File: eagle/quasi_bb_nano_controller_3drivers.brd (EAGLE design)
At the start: 62.4 x 70.6 mm, 10 parts, among them X1 JST-XH-08-PIN-LONG-PAD, X2 JST-XH-08-PIN-LONG-PAD, X3 JST-XH-02-PIN-LONG-PAD, X4 JST-XH-08-PIN-LONG-PAD, X5 JST-XH-08-PIN-LONG-PAD

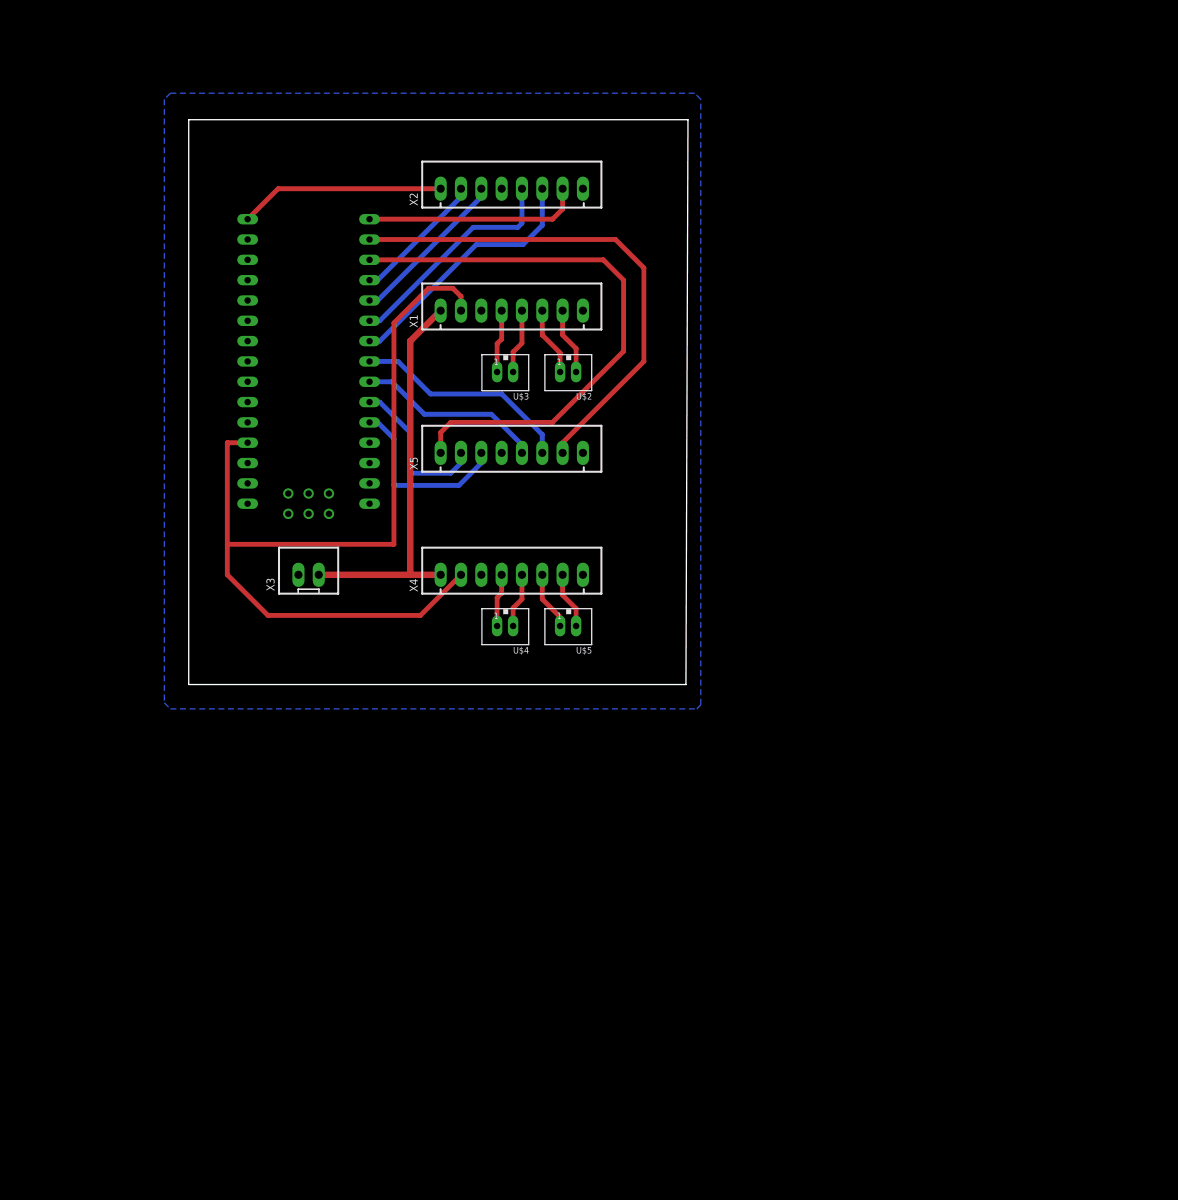
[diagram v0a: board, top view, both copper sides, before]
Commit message: Add eagle
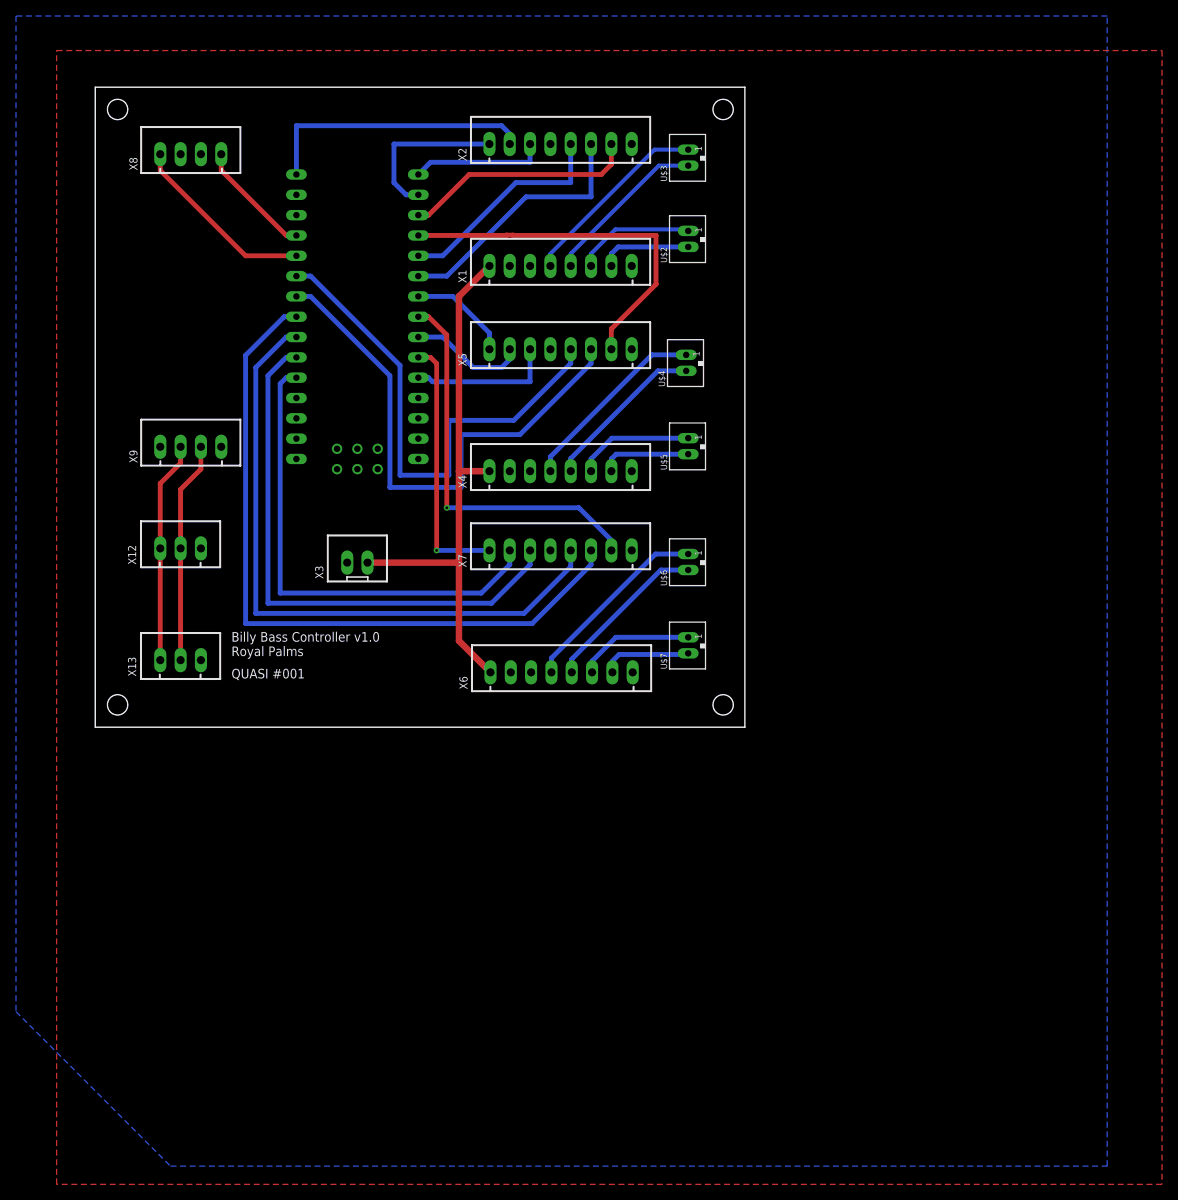
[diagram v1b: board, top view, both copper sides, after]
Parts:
- added U$6, U$7: JST-PH_2-PIN_HEADER, con-jst-ph:JST_B2B-PH_HEADER
- added X12, X13: JST-XH-03-PIN-LONG-PAD, Rembrandt Electronics - JST XH Connectors v1-0:JST-XH-03-PACKAGE-LONG-PAD
- added X6, X7: JST-XH-08-PIN-LONG-PAD, Rembrandt Electronics - JST XH Connectors v1-0:JST-XH-08-PACKAGE-LONG-PAD
- added X8, X9: JST-XH-04-PIN-LONG-PAD, Rembrandt Electronics - JST XH Connectors v1-0:JST-XH-04-PACKAGE-LONG-PAD
- moved U$4 39.8 mm to (73.9, 45.5), turned to 90 degrees
- moved U$3 35.1 mm to (74.2, 71.1), turned to 90 degrees
- moved U$5 26.9 mm to (74.2, 35.1), turned to 90 degrees
- moved U$2 22.3 mm to (74.2, 61.0), turned to 90 degrees
- moved X5 14.3 mm to (58.2, 47.2)
- moved X4 14.3 mm to (58.2, 32.0)
- moved U$1 8.27 mm to (35.3, 42.4)
- moved X1 8.27 mm to (58.2, 57.7)
- moved X2 8.27 mm to (58.2, 72.9)
- moved X3 6.28 mm to (32.8, 20.6)
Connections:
- removed net N$12: X2.4
- removed net N$121: X5.4
- new net 485_A: X12.1, X13.1, X9.2
- new net 485_B: X12.2, X13.2, X9.3
- new net A0: U$1.A0, X8.4
- new net A01_2: U$6.P1, X6.4
- new net A02_2: U$6.P2, X6.5
- new net A1: U$1.A1, X8.1
- new net A1_2: U$1.A6, X7.3
- new net A2_2: U$1.A7, X7.2
- new net B01_2: U$7.P2, X6.7
- new net B02_2: U$7.P1, X6.6
- new net B1_2: U$1.A5, X7.5
- new net B2_2: U$1.A4, X7.6
- new net PWMA_2: U$1.D3, X7.1
- new net PWMB_2: U$1.D5, X7.7
- net A1_0: now also U$1.D12; no longer U$1.D8
- net A2_0: now also U$1.D13; no longer U$1.D9
- net A2_1: now also U$1.D4; no longer U$1.D3
- net B1_0: now also U$1.D8; no longer U$1.D7
- net B1_1: now also U$1.A2; no longer U$1.D4
- net B2_0: now also U$1.D7; no longer U$1.D6
- net B2_1: now also U$1.A3; no longer U$1.D5
- net GND: now also X12.3, X13.3, X6.3, X6.8, X7.8, X8.2, X8.3, X9.1
- net PWMA_0: now also U$1.D11; no longer U$1.D13
- net PWMA_1: now also U$1.D6; no longer U$1.D10
- net PWMB_0: now also U$1.D10; no longer U$1.D12
- net PWMB_1: now also U$1.D9; no longer U$1.D11
- net VCC: now also X6.2, X9.4
- net VM: now also X6.1
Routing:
- net VCC: track 129.9 -> 0.00 mm
- net B2_2: track 0.00 -> 89.9 mm
- net B1_2: track 0.00 -> 81.2 mm
- net A1_2: track 0.00 -> 69.5 mm
- net A2_2: track 0.00 -> 60.5 mm
- net PWMA_1: track 71.3 -> 12.8 mm
- net PWMB_2: track 0.00 -> 49.6 mm, vias 0 -> 1
- net B1_1: track 23.3 -> 64.2 mm
- net B2_1: track 27.7 -> 67.0 mm
- net PWMA_2: track 0.00 -> 32.6 mm, vias 0 -> 1
- net 485_B: track 0.00 -> 27.7 mm
- net 485_A: track 0.00 -> 27.7 mm
- net A01_2: track 0.00 -> 24.3 mm
- net A1: track 0.00 -> 23.5 mm
- net A02_2: track 0.00 -> 20.8 mm
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- added copper zone on layer 1, net VCC
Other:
- board size 62.4 x 70.6 mm -> 81.2 x 80 mm
- board text added: "Billy Bass Controller v1.0 Royal Palms"
- board text added: "QUASI #001"
